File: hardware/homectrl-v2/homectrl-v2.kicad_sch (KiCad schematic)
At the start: 96 parts, among them J1 Barrel_Jack, J2 PUMP1_CONN, J3 PUMP2_CONN, J4 STEP_CONN, J5 USB_C_CONN, J6 SMS1_CONN, J7 SMS2_CONN, J8 FSW1_CONN, J9 FSW2_CONN, Q1 DMP6023LE-13, Q2 2N7002, Q3 PMOS, Q4 PMOS, Q5 AO3400A, SW1 S3_RESET_SW, SW2 S3_BOOT_SW, U1 TPS5405DR, U2 AMS1117-3.3, U3 DMP4065S-7, U4 ESP32-S3-WROOM-1, U5 TMC2209, U6 ADS1115IDGS, U8 TPD2E001DRLR, U9 TPD2E001DRLR

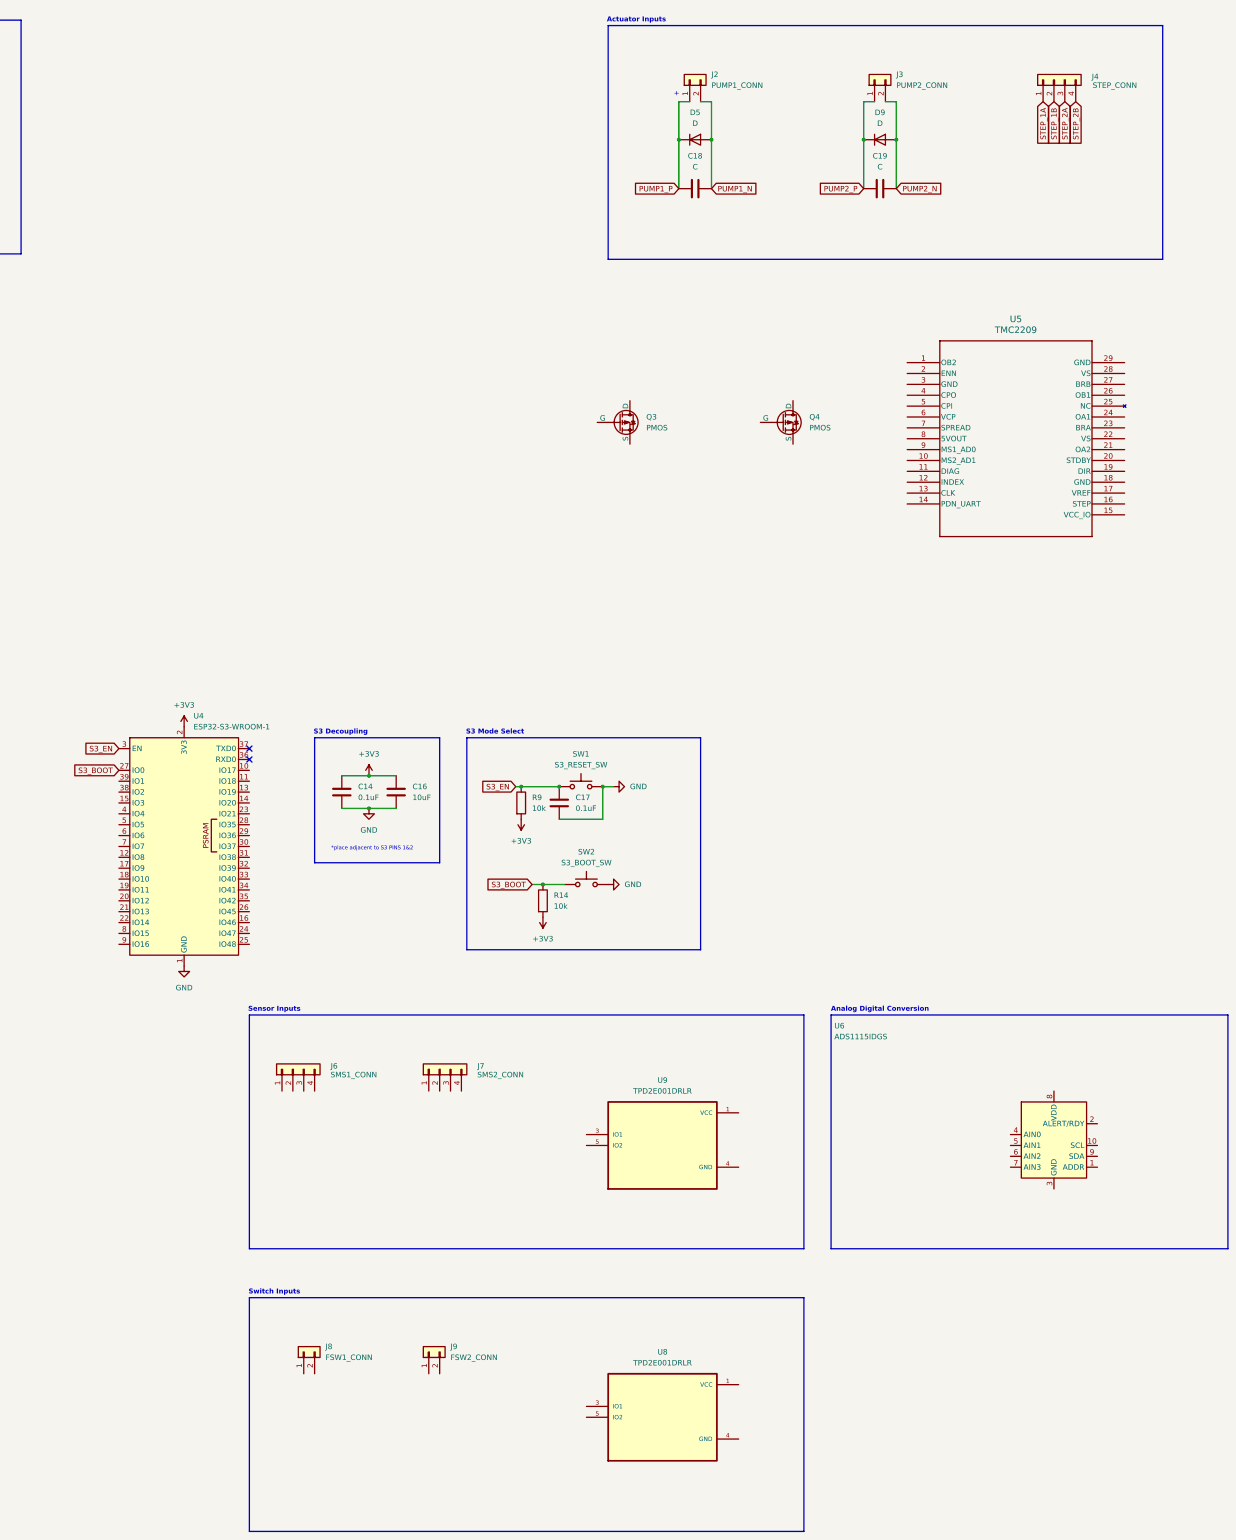
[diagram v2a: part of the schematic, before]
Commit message: peirpheral circuit work
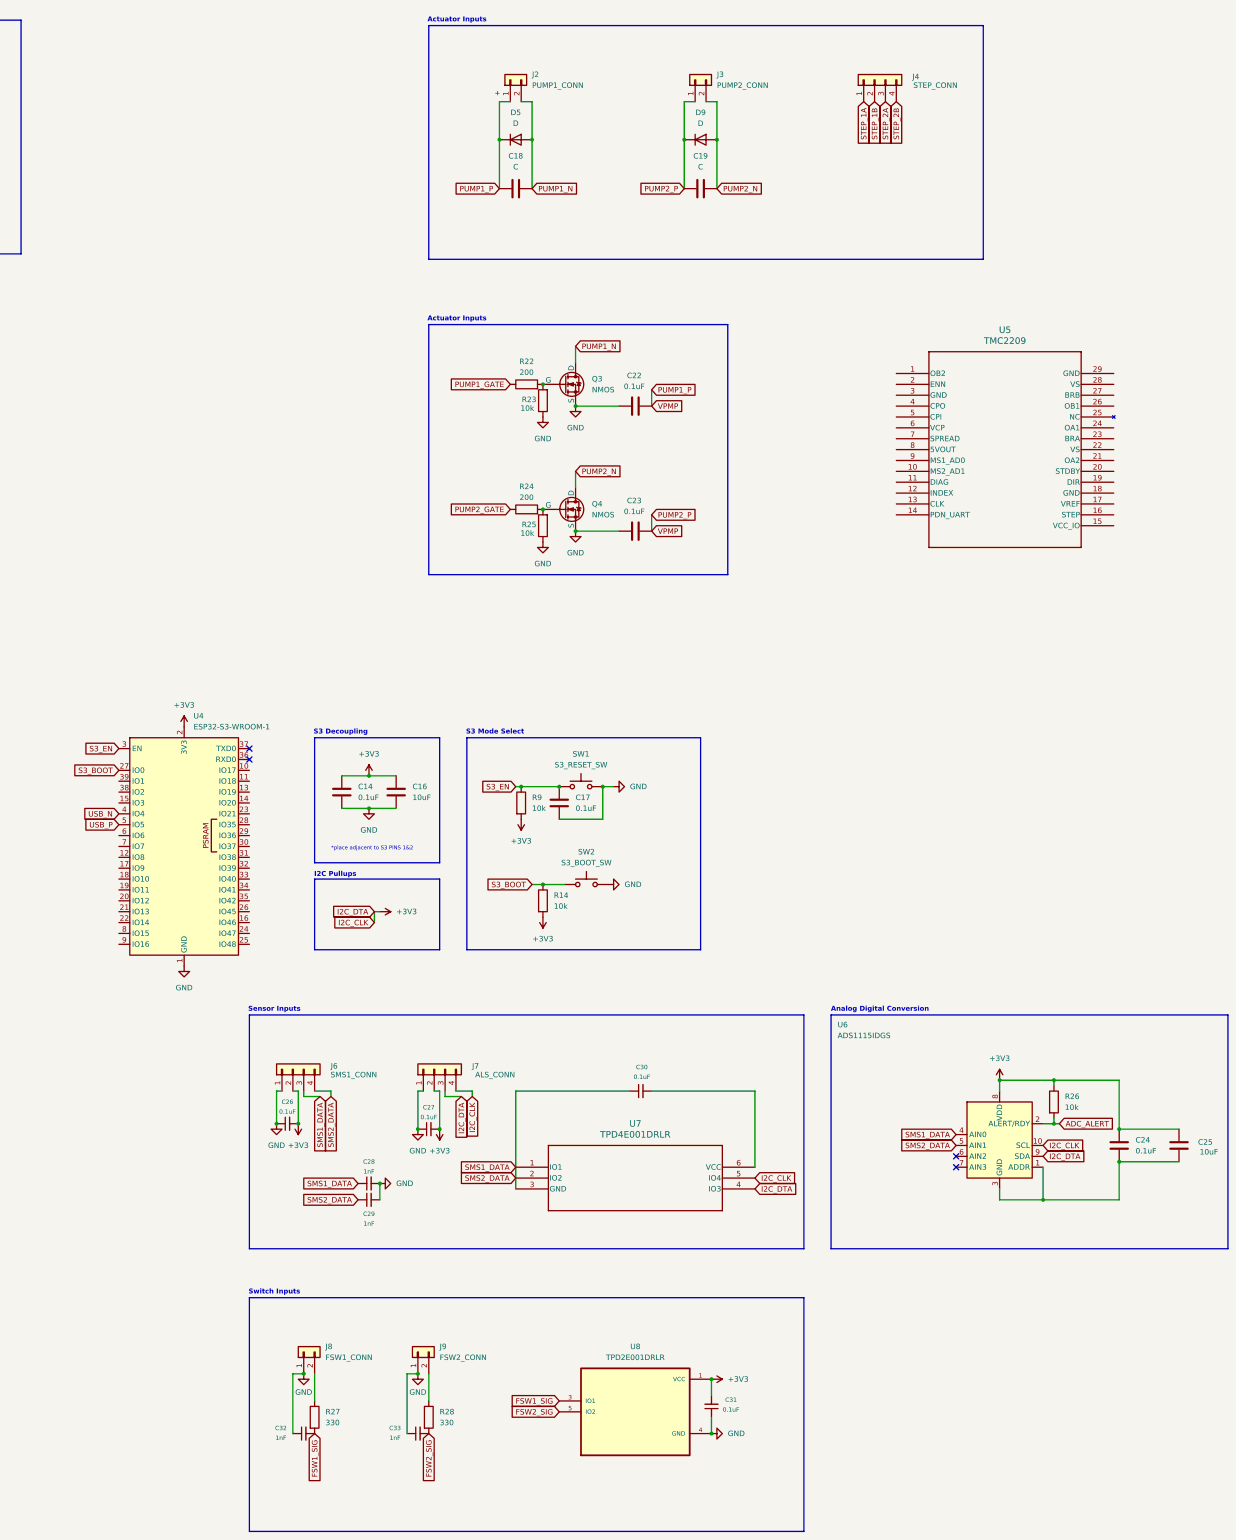
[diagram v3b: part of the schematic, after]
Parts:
- removed Q3, Q4: PMOS, symbol Simulation_SPICE:PMOS
- removed U9: TPD2E001DRLR, TPD2E001DRLR:SOT50P160X60-5N, symbol TPD2E001DRLR:TPD2E001DRLR
- added C22, C23, C24: 0.1uF, Capacitor_SMD:C_0402_1005Metric, symbol Device:C
- added C25: 10uF, Capacitor_SMD:C_0805_2012Metric, symbol Device:C
- added C26, C27, C30, C31: 0.1uF, Capacitor_SMD:C_0402_1005Metric, symbol Device:C_Small
- added C28, C29, C32, C33: 1nF, Capacitor_SMD:C_0402_1005Metric, symbol Device:C_Small
- added Q3, Q4: NMOS, symbol Simulation_SPICE:NMOS
- added R22, R24: 200, Resistor_SMD:R_0402_1005Metric, symbol Device:R
- added R23, R25: 10k, Resistor_SMD:R_0603_1608Metric, symbol Device:R
- added R26: 10k, Resistor_SMD:R_0402_1005Metric, symbol Device:R
- added R27, R28: 330, Resistor_SMD:R_0402_1005Metric, symbol Device:R
- added U7: TPD4E001DRLR, DRL6, symbol TPD4E001DRLR:TPD4E001DRLR
- J7: value SMS2_CONN -> ALS_CONN
- R13: footprint Resistor_SMD:R_0603_1608Metric -> Resistor_SMD:R_0402_1005Metric
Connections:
- net PUMP2_P is gone; now on net PUMP1_P: C19.1, D9.1 (K), J3.1 (Pin_1)
- net VPMP is gone; now on net PUMP1_P: R15.2, U3.3 (D)
- net +3V3: now also J6.2 (Pin_2), J7.2 (Pin_2), J7.3 (Pin_3), J7.4 (Pin_4), U6.10 (SCL), U6.8 (VDD), U6.9 (SDA), U8.1 (VCC), C24.1, C25.2, C26.2, C27.2, C31.2, R26.1, U7.4 (IO3), U7.5 (IO4)
- net GND: now also J6.1 (Pin_1), J7.1 (Pin_1), J8.1 (Pin_1), J9.1 (Pin_1), U8.4 (GND), C22.2, C23.2, C26.1, C27.1, C28.2, C29.2, C31.1, C32.1, C33.1, Q3.3 (S), Q4.3 (S), R23.1, R25.1
- net PUMP1_N: now also Q3.1 (D)
- net PUMP1_P: now also C22.1, C23.1
- net PUMP2_N: now also Q4.1 (D)
- net USB_N: now also U4.4 (IO4)
- net USB_P: now also U4.5 (IO5)
- net at U6.1 (ADDR): now also U6.3 (GND), C24.2, C25.1
- net ADC_ALERT: now reaches U6.2 (ALERT/RDY)
- net ADC_ALERT: now also R26.2
- net SMS1_DATA: now reaches U6.4 (AIN0)
- net SMS1_DATA: now also J6.3 (Pin_3), J6.4 (Pin_4), U6.5 (AIN1), C28.1, C29.1, C30.1, U7.1 (IO1), U7.2 (IO2), U7.3 (GND)
- net at J9.2 (Pin_2): now also R28.1
- net at J8.2 (Pin_2): now also R27.1
- net FSW1_SIG: now reaches U8.3 (IO1)
- net FSW1_SIG: now also C32.2, R27.2
- net FSW2_SIG: now reaches U8.5 (IO2)
- net FSW2_SIG: now also C33.2, R28.2
- new net: C30.2, U7.6 (VCC)
- new net: Q3.2 (G), R22.2, R23.2
- new net: Q4.2 (G), R24.2, R25.2
- new net PUMP1_GATE: R22.1
- new net PUMP2_GATE: R24.1
- no-connect marks 5 -> 7
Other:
- note added: "I2C Pullups"
- moved on the sheet: C18, C19, D5, D9, J2, J3, J4, U5, U6, U8

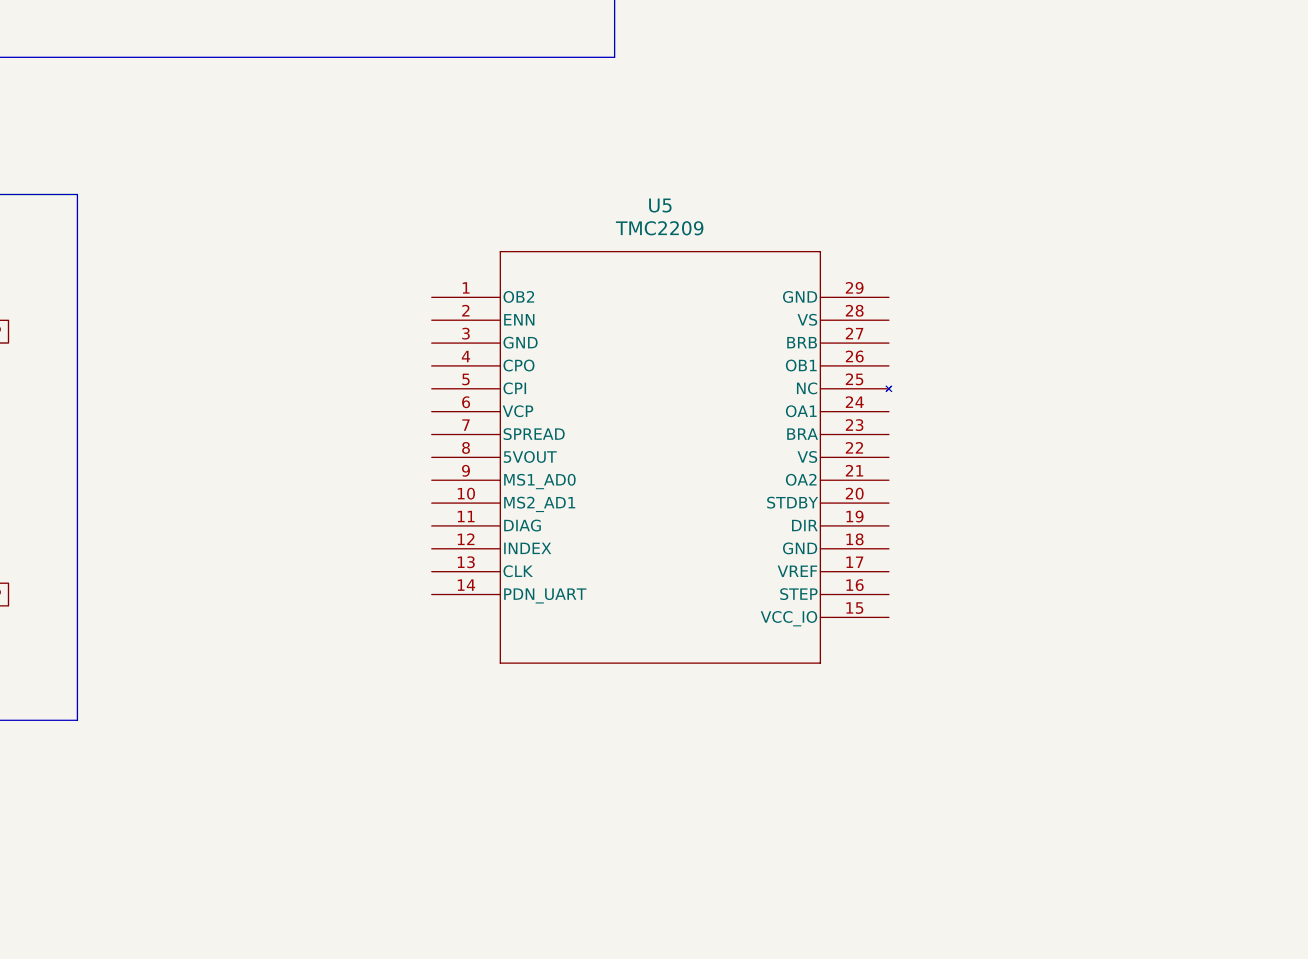
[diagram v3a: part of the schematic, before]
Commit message: tmc2209 wiring
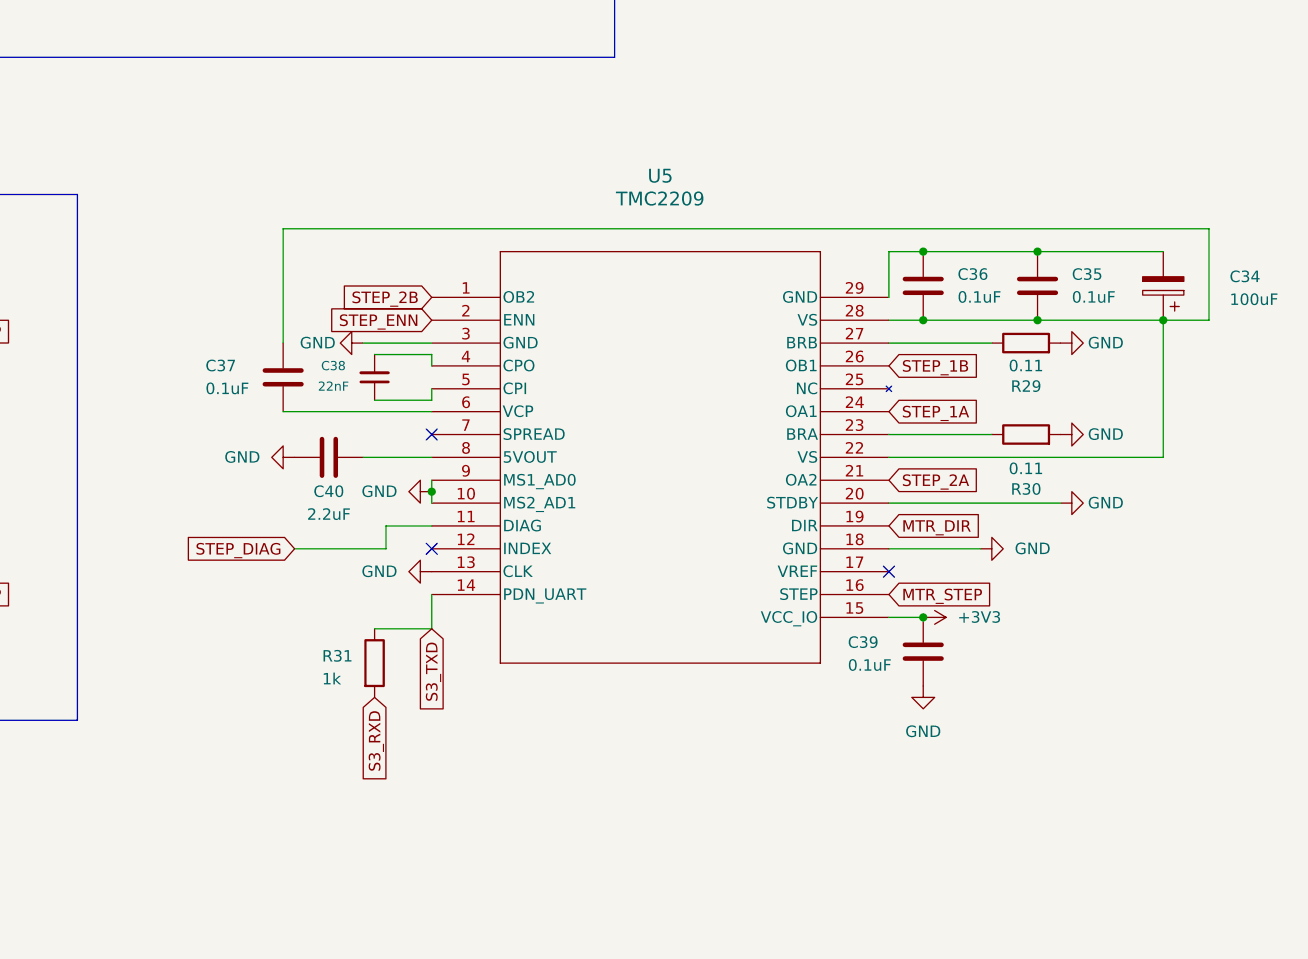
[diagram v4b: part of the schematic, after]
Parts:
- added C34: 100uF, symbol Device:C_Polarized
- added C35, C36, C37, C39: 0.1uF, Capacitor_SMD:C_0402_1005Metric, symbol Device:C
- added C38: 22nF, Capacitor_SMD:C_0402_1005Metric, symbol Device:C_Small
- added C40: 2.2uF, symbol Device:C
- added R29: 0.11, Resistor_SMD:R_0402_1005Metric, symbol Device:R
- added R30: 0.11, symbol Device:R
- added R31: 1k, Resistor_SMD:R_0402_1005Metric, symbol Device:R
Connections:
- net +3V3: now also U5.15 (VCC_IO), C39.1
- net GND: now also U5.10 (MS2_AD1), U5.13 (CLK), U5.18 (GND), U5.20 (STDBY), U5.3 (GND), U5.9 (MS1_AD0), C39.2, C40.1, R29.2, R30.2
- net STEP_1A: now also U5.24 (OA1)
- net STEP_1B: now also U5.26 (OB1)
- net STEP_2A: now also U5.21 (OA2)
- net STEP_2B: now also U5.1 (OB2)
- net STEP_DIAG: now reaches U5.11 (DIAG)
- net S3_TXD: now reaches U5.14 (PDN_UART)
- net S3_TXD: now also R31.1
- net MTR_STEP: now reaches U5.16 (STEP)
- net MTR_DIR: now reaches U5.19 (DIR)
- net STEP_ENN: now reaches U5.2 (ENN)
- net at U5.22 (VS): now also U5.28 (VS), C34.1, C35.2, C36.2, C37.1
- net at U5.23 (BRA): now also R30.1
- net at U5.27 (BRB): now also R29.1
- net at U5.29 (GND): now also C34.2, C35.1, C36.1
- net at U5.4 (CPO): now also C38.2
- net at U5.5 (CPI): now also C38.1
- net at U5.6 (VCP): now also C37.2
- net at U5.8 (5VOUT): now also C40.2
- new net S3_RXD: R31.2
- no-connect marks 7 -> 10
